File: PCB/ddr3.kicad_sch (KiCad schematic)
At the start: 34 parts, among them U11 MT41J128M16JT-125:K

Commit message: even more footprints
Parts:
- C110, C86: footprint (none) -> Capacitor_SMD:C_0402_1005Metric
- C85: footprint (none) -> Capacitor_SMD:C_1206_3216Metric
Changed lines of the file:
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@@
 			)
 		)
-		(property "Footprint" ""
+		(property "Footprint" "Capacitor_SMD:C_0402_1005Metric"
 			(at 176.2252 201.93 0)
 			(effects
@@
 			)
 		)
-		(property "Footprint" ""
+		(property "Footprint" "Capacitor_SMD:C_1206_3216Metric"
 			(at 387.0452 128.27 0)
 			(effects
@@
 			)
 		)
-		(property "Footprint" ""
+		(property "Footprint" "Capacitor_SMD:C_0402_1005Metric"
 			(at 176.2252 191.77 0)
 			(effects

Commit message: fixing a bunch of footprints to standardize
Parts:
- C75: footprint Capacitor_SMD:C_0603_1608Metric -> Capacitor_SMD:C_1206_3216Metric
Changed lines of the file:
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@@
 			)
 		)
-		(property "Footprint" "Capacitor_SMD:C_0603_1608Metric"
+		(property "Footprint" "Capacitor_SMD:C_1206_3216Metric"
 			(at 177.4952 128.27 0)
 			(effects

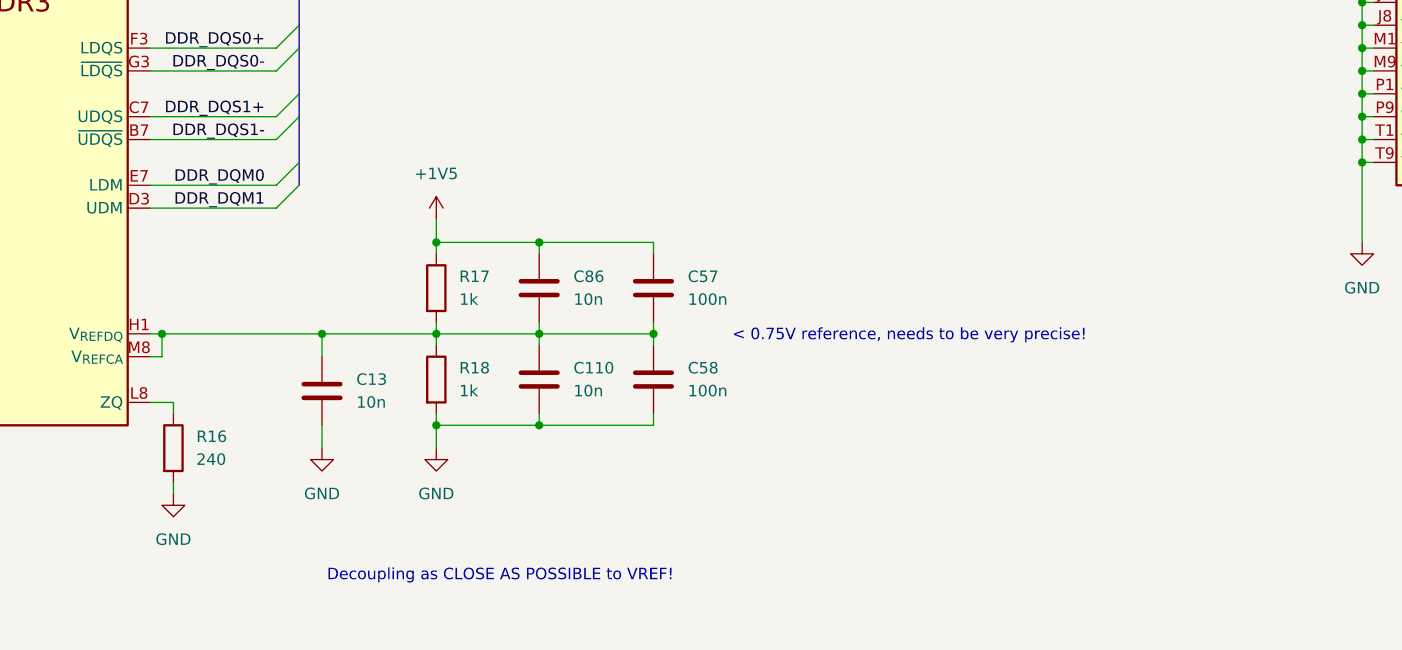
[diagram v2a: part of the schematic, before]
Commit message: fixing my  VREF decoupling, starting to route it!
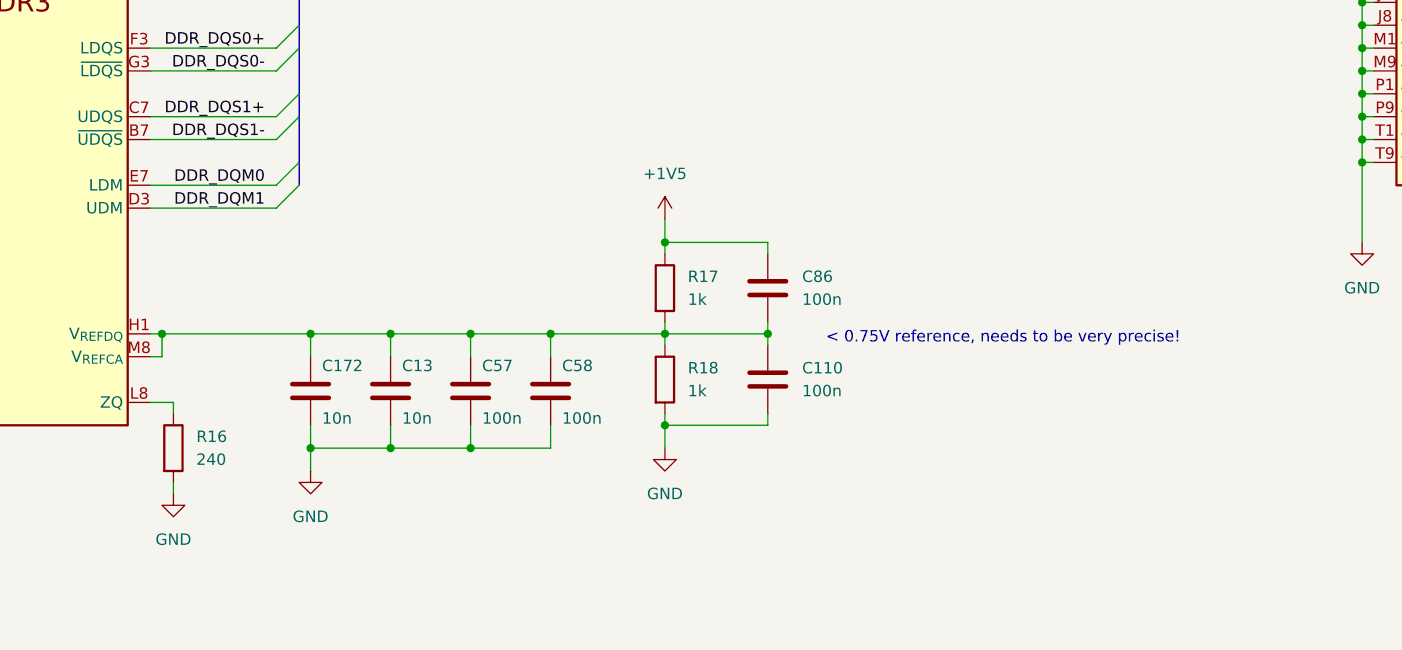
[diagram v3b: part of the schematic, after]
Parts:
- removed C110, C86: 10n, Capacitor_SMD:C_0402_1005Metric, symbol Device:C
- added C172: 10n, Capacitor_SMD:C_0402_1005Metric, symbol Device:C
- added C57, C58: 100n, Capacitor_SMD:C_0402_1005Metric, symbol Device:C
- renumbered C58 to C110, C57 to C86
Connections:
- net GND: now also C172.2, C57.2, C58.2
- net at C110.1, C13.1, C86.2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: now also C172.1, C57.1, C58.1
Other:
- note removed: "Decoupling as CLOSE AS POSSIBLE to VREF!"
- moved on the sheet: C110, C86, R17, R18

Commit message: fixing my pads
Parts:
- U11: footprint Package_BGA:Micron_FBGA-96_8x14mm_Layout9x16_P0.8mm -> FPGA:FBGA-96_8x14mm_Layout9x16_P0.8mm
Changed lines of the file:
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@@
 			)
 		)
-		(property "Footprint" "Package_BGA:Micron_FBGA-96_8x14mm_Layout9x16_P0.8mm"
+		(property "Footprint" "FPGA:FBGA-96_8x14mm_Layout9x16_P0.8mm"
 			(at 116.84 213.614 0)
 			(effects
@@
 			)
 		)
-		(property "Footprint" "Package_BGA:Micron_FBGA-96_8x14mm_Layout9x16_P0.8mm"
+		(property "Footprint" "FPGA:FBGA-96_8x14mm_Layout9x16_P0.8mm"
 			(at 283.21 186.944 0)
 			(effects
